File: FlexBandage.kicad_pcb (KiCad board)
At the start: 2 copper layers, 79.7 x 19 mm, 34 parts, among them J1 FFC3B07-04-T, U1 ESP32-C3FH4, U2 MCP73831-2-OT, U3 TMP117, U4 MIC5504-3.3YMT-T5, Y1 ECS-400-10-37B-CKY-TR3

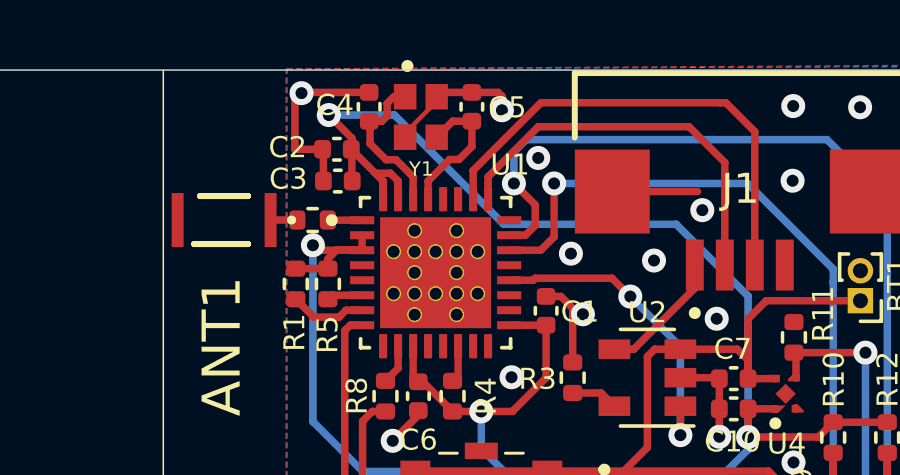
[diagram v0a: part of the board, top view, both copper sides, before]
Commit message: update badge
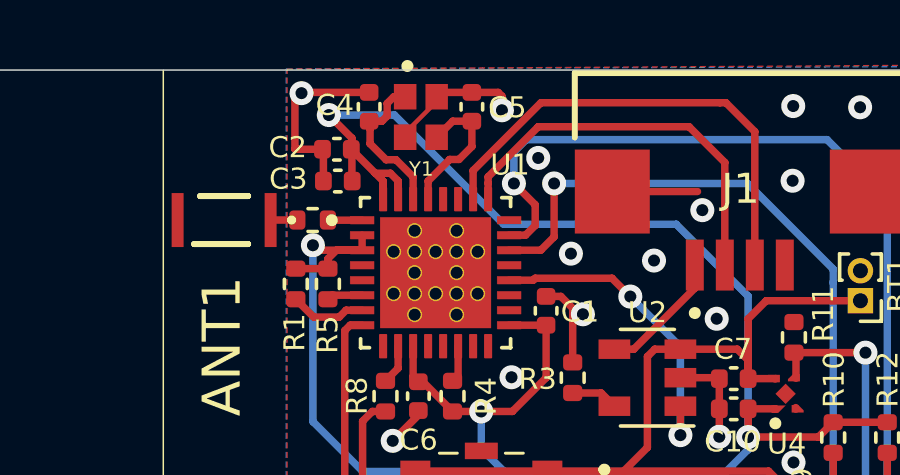
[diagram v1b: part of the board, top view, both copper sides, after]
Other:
- board text added: "STIFFENER"
